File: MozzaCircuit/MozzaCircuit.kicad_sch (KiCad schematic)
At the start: 17 parts, among them J1 8P8C_both_sides, U1 MCP23017_ML, U2 MCP23017_ML_NoTP

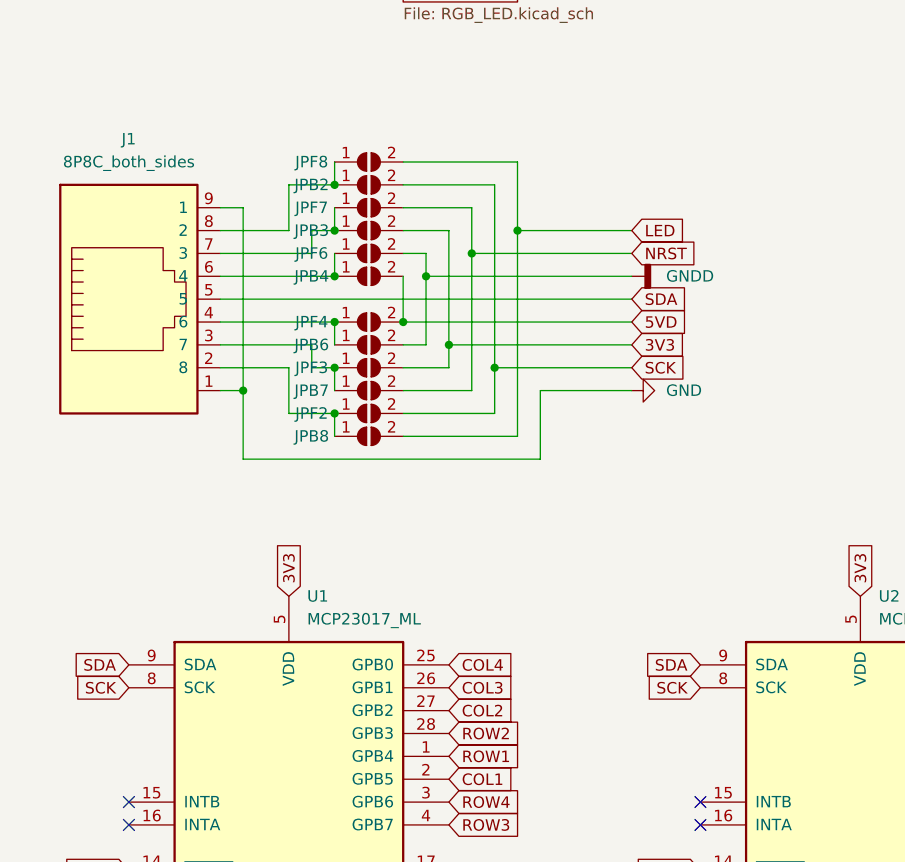
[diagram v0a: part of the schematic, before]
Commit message: rj45 wiring
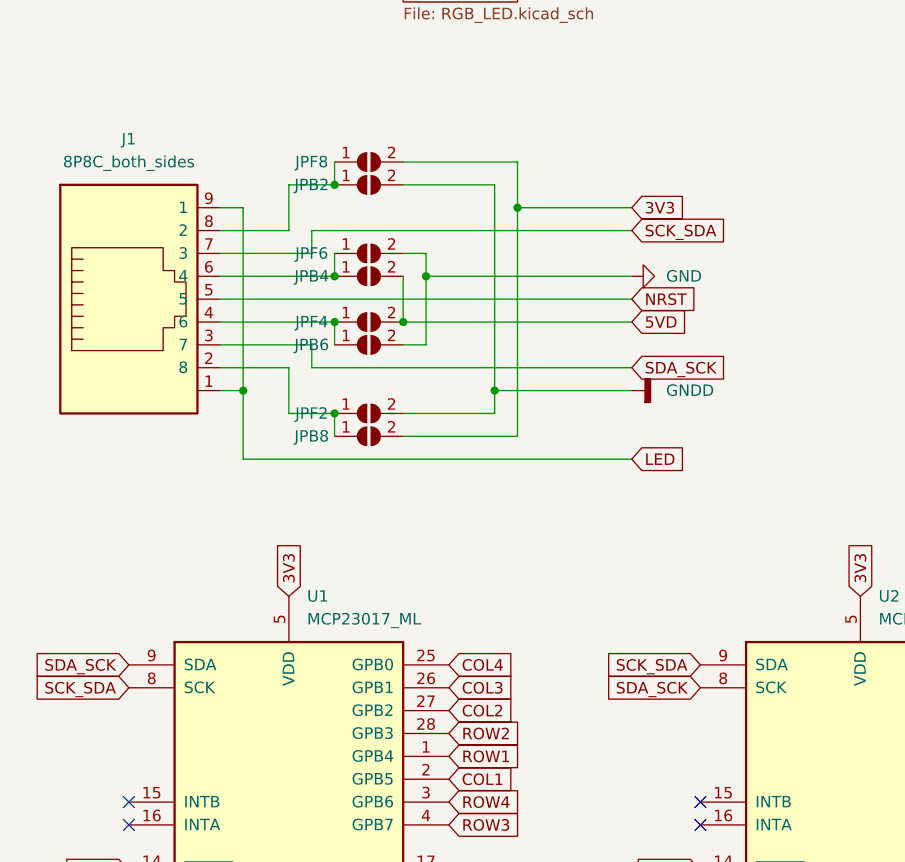
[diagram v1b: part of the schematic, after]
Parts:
- removed JPB3, JPB7, JPF3, JPF7: SolderJumper_2_Open, Jumper:SolderJumper-2_P1.3mm_Open_TrianglePad1.0x1.5mm, symbol Jumper:SolderJumper_2_Open
- JPB2, JPB4, JPB6, JPB8, JPF2, JPF4, JPF6, JPF8: footprint Jumper:SolderJumper-2_P1.3mm_Open_TrianglePad1.0x1.5mm -> 00_KeyParts:SolderJumper-2_P1.3mm_Open_TrianglePad1.0x1.5mm
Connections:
- net 3V3: now also JPB8.2 (B), JPF8.2 (B)
- net GND: now also JPB6.2 (B), JPF6.2 (B); no longer J1.1, J1.9 (1)
- net GNDD: now also JPB2.2 (B), JPF2.2 (B); no longer JPB6.2 (B), JPF6.2 (B)
- net LED: now also J1.1, J1.9 (1); no longer JPB8.2 (B), JPF8.2 (B)
- net NRST: now also J1.5
- net SCK_SDA: now reaches J1.7 (3)
- net SCK_SDA: now also U1.8 (SCK), U2.9 (SDA)
- net SDA_SCK: now reaches J1.3 (7)
- net SDA_SCK: now also U1.9 (SDA), U2.8 (SCK)
- removed net SCK: JPB2.2 (B), JPF2.2 (B), U1.8 (SCK), U2.8 (SCK)
- removed net SDA: J1.5, U1.9 (SDA), U2.9 (SDA)
